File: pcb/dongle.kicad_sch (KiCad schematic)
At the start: 33 parts, among them J1 USB_A, J2 Conn_01x01_Pin, J3 Conn_01x01_Pin, J4 Conn_01x01_Pin, J5 Conn_01x01_Pin, SW1 SW_Push_45deg, U3 nRF52833_QDxx, Y1 Crystal_GND24, Y2 Crystal_Small

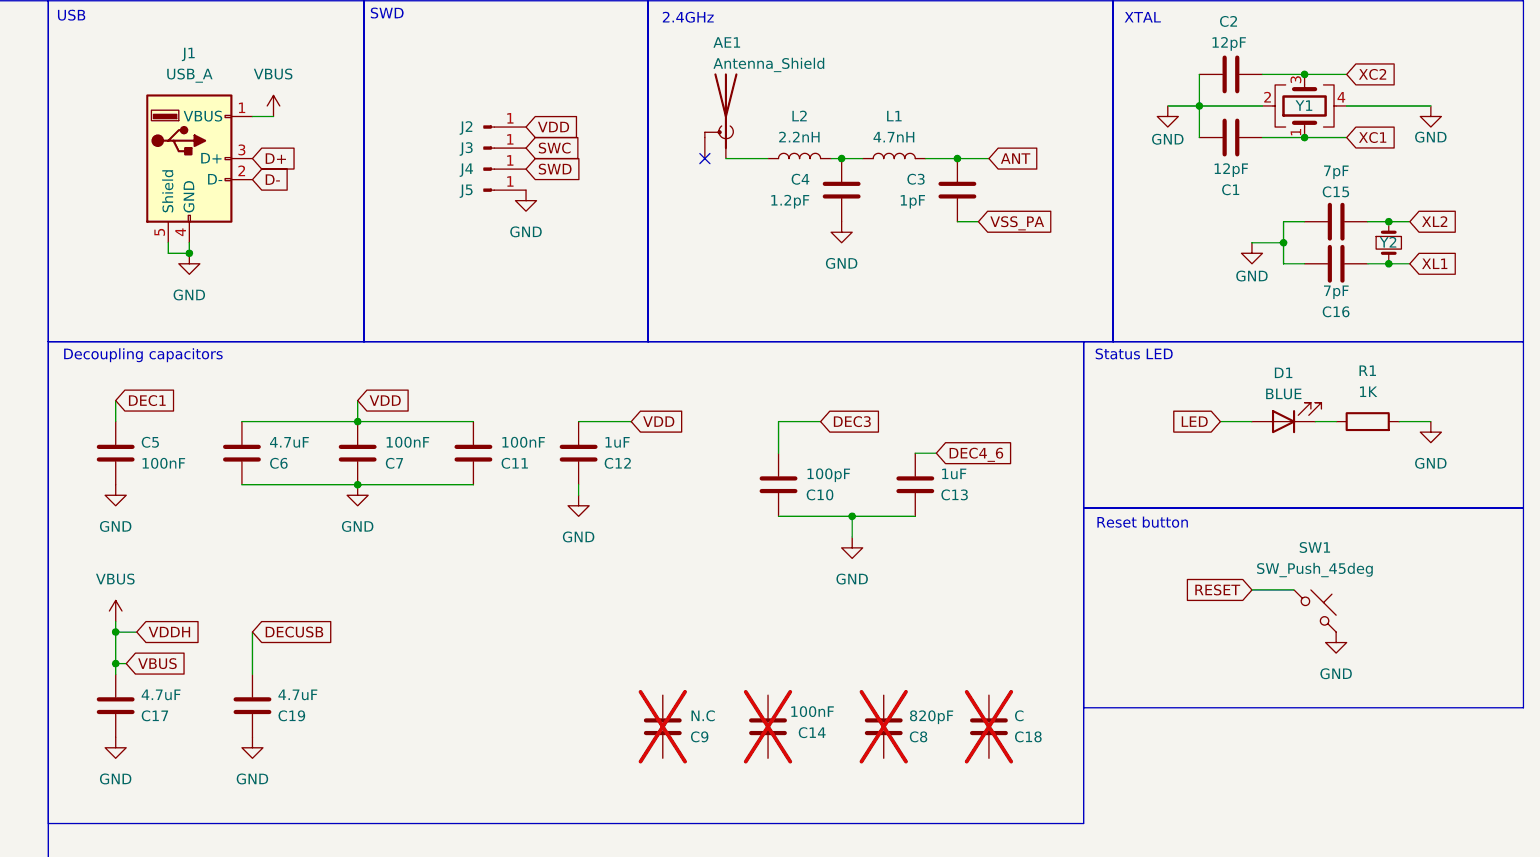
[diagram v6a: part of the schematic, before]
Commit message: update pcb
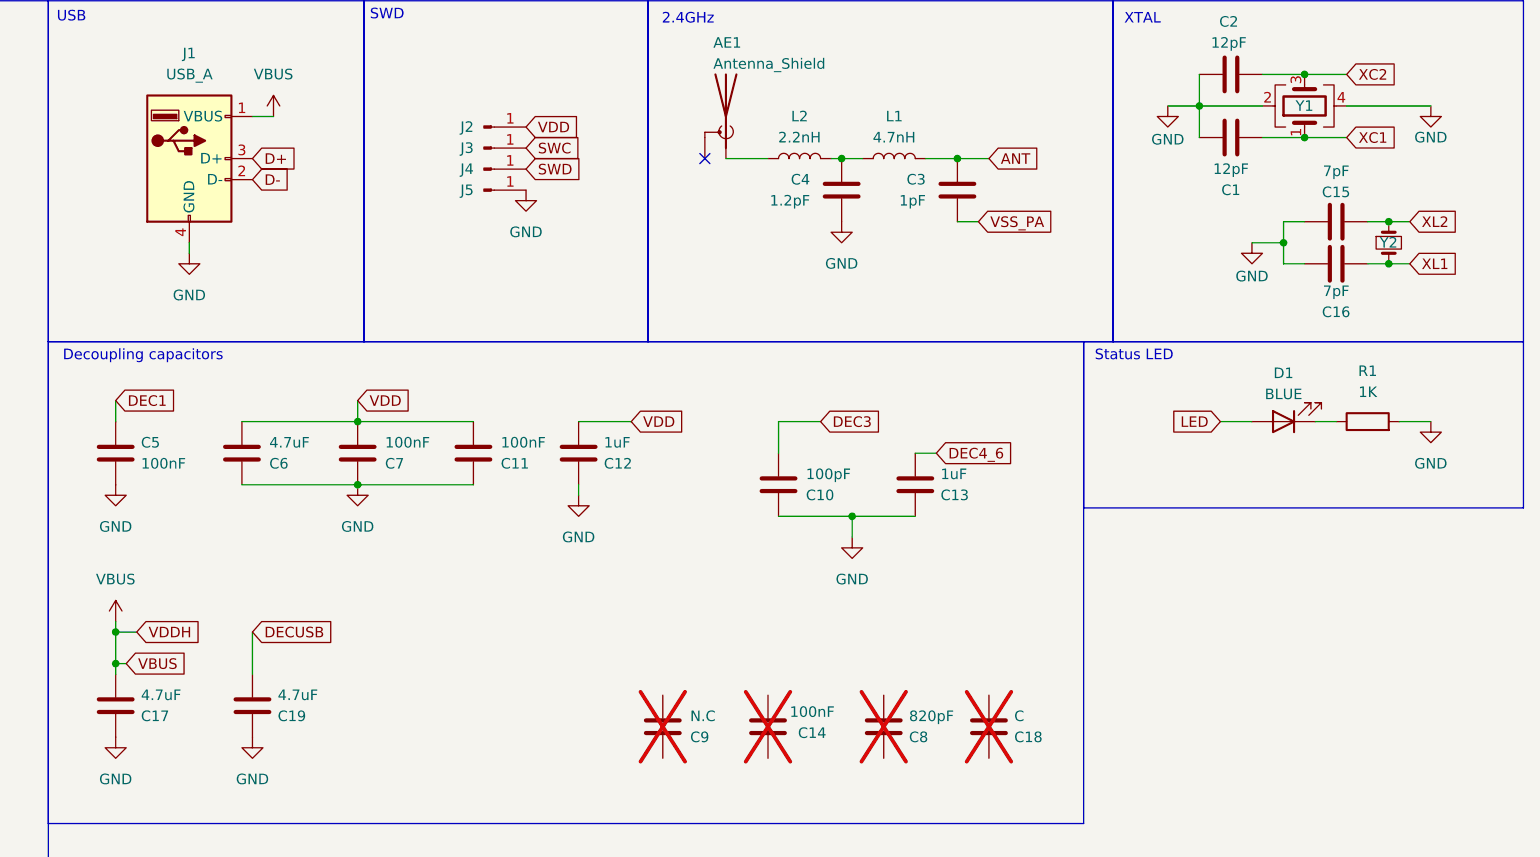
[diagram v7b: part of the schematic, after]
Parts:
- removed SW1: SW_Push_45deg, dongle:SW_SPST_B3U-1000P, symbol dongle:SW_Push_45deg
- J1: footprint dongle:USB_A_Molex_48037-2200_Horizontal -> dongle:USB_A_PCB_Edge_receptacle
- U3: footprint dongle:QFN-40-1EP_5x5mm_P0.4mm_EP3.6x3.6mm_ThermalVias -> dongle:QFN-40-1EP_5x5mm_P0.4mm_EP3.6x3.6mm
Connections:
- net GND: no longer J1.5 (Shield)
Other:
- note removed: "Reset button"
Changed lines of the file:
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@@
 		)
 	)
-	(rectangle
-		(start 231.14 73.914)
-		(end 284.226 98.044)
-		(stroke
-			(width 0)
-			(type default)
-		)
-		(fill
-			(type none)
-		)
-	)
 	(text "USB"
 		(exclude_from_sim no)
@@
 		)
 	)
-	(text "Reset button"
-		(exclude_from_sim no)
-		(at 238.252 75.946 0)
-		(effects
-			(font
-				(size 1.27 1.27)
-			)
-		)
-	)
 	(text "XTAL"
 		(exclude_from_sim no)
@@
 	)
 	(junction
-		(at 123.19 43.18)
-		(diameter 0)
-		(color 0 0 0 0)
-	)
-	(junction
 		(at 267.97 39.37)
 		(diameter 0)
@@
 	(wire
 		(pts
-			(xy 120.65 43.18) (xy 123.19 43.18)
-		)
-		(stroke
-			(width 0)
-			(type default)
-		)
-	)
-	(wire
-		(pts
 			(xy 245.11 25.4) (xy 252.73 25.4)
 		)
@@
 	(wire
 		(pts
-			(xy 251.46 83.82) (xy 256.54 83.82)
-		)
-		(stroke
-			(width 0)
-			(type default)
-		)
-	)
-	(wire
-		(pts
 			(xy 187.96 31.75) (xy 193.04 31.75)
 		)
@@
 	(wire
 		(pts
-			(xy 120.65 41.91) (xy 120.65 43.18)
-		)
-		(stroke
-			(width 0)
-			(type default)
-		)
-	)
-	(wire
-		(pts
 			(xy 115.57 92.71) (xy 114.3 92.71)
 		)
@@
 		)
 	)
-	(global_label "RESET"
-		(shape input)
-		(at 251.46 83.82 180)
-		(fields_autoplaced yes)
-		(effects
-			(font
-				(size 1.27 1.27)
-			)
-			(justify right)
-		)
-		(property "Intersheetrefs" "${INTERSHEET_REFS}"
-			(at 242.7297 83.82 0)
-			(effects
-				(font
-					(size 1.27 1.27)
-				)
-				(justify right)
-				(hide yes)
-			)
-		)
-	)
 	(global_label "VDD"
 		(shape input)
@@
 	)
 	(symbol
-		(lib_id "dongle:SW_Push_45deg")
-		(at 259.08 86.36 0)
-		(unit 1)
-		(exclude_from_sim no)
-		(in_bom yes)
-		(on_board yes)
-		(dnp no)
-		(fields_autoplaced yes)
-		(property "Reference" "SW1"
-			(at 259.08 78.74 0)
-			(effects
-				(font
-					(size 1.27 1.27)
-				)
-			)
-		)
-		(property "Value" "SW_Push_45deg"
-			(at 259.08 81.28 0)
-			(effects
-				(font
-					(size 1.27 1.27)
-				)
-			)
-		)
-		(property "Footprint" "dongle:SW_SPST_B3U-1000P"
-			(at 259.08 86.36 0)
-			(effects
-				(font
-					(size 1.27 1.27)
-				)
-				(hide yes)
-			)
-		)
-		(property "Datasheet" "~"
-			(at 259.08 86.36 0)
-			(effects
-				(font
-					(size 1.27 1.27)
-				)
-				(hide yes)
-			)
-		)
-		(property "Description" "Push button switch, normally open, two pins, 45° tilted"
-			(at 259.08 86.36 0)
-			(effects
-				(font
-					(size 1.27 1.27)
-				)
-				(hide yes)
-			)
-		)
-		(pin "2"
-		)
-		(pin "1"
-		)
-		(instances
-			(project ""
-				(path "/81b8789c-509b-48aa-aabd-6327c54a25df"
-					(reference "SW1")
-					(unit 1)
-				)
-			)
-		)
-	)
-	(symbol
 		(lib_id "PNCATEHO_lowair:C")
 		(at 170.18 67.31 0)
@@
 	)
 	(symbol
-		(lib_id "Library:GND")
-		(at 261.62 88.9 0)
-		(unit 1)
-		(exclude_from_sim no)
-		(in_bom yes)
-		(on_board yes)
-		(dnp no)
-		(fields_autoplaced yes)
-		(property "Reference" "#PWR05"
-			(at 261.62 95.25 0)
-			(effects
-				(font
-					(size 1.27 1.27)
-				)
-				(hide yes)
-			)
-		)
-		(property "Value" "GND"
-			(at 261.62 93.98 0)
-			(effects
-				(font
-					(size 1.27 1.27)
-				)
-			)
-		)
-		(property "Footprint" ""
-			(at 261.62 88.9 0)
-			(effects
-				(font
-					(size 1.27 1.27)
-				)
-				(hide yes)
-			)
-		)
-		(property "Datasheet" ""
-			(at 261.62 88.9 0)
-			(effects
-				(font
-					(size 1.27 1.27)
-				)
-				(hide yes)
-			)
-		)
-		(property "Description" "Global ground symbol"
-			(at 261.62 98.298 0)
-			(effects
-				(font
-					(size 1.27 1.27)
-				)
-				(hide yes)
-			)
-		)
-		(pin "1"
-		)
-		(instances
-			(project "dongle"
-				(path "/81b8789c-509b-48aa-aabd-6327c54a25df"
-					(reference "#PWR05")
-					(unit 1)
-				)
-			)
-		)
-	)
-	(symbol
 		(lib_id "PNCATEHO_lowair:VBUS")
 		(at 114.3 87.63 0)
@@
 			)
 		)
-		(property "Footprint" "dongle:USB_A_Molex_48037-2200_Horizontal"
+		(property "Footprint" "dongle:USB_A_PCB_Edge_receptacle"
 			(at 127 33.02 0)
 			(effects
@@
 		(pin "1"
 		)
-		(pin "5"
-		)
 		(instances
 			(project ""
@@
 			)
 		)
-		(property "Footprint" "dongle:QFN-40-1EP_5x5mm_P0.4mm_EP3.6x3.6mm_ThermalVias"
+		(property "Footprint" "dongle:QFN-40-1EP_5x5mm_P0.4mm_EP3.6x3.6mm"
 			(at 59.69 180.34 0)
 			(effects

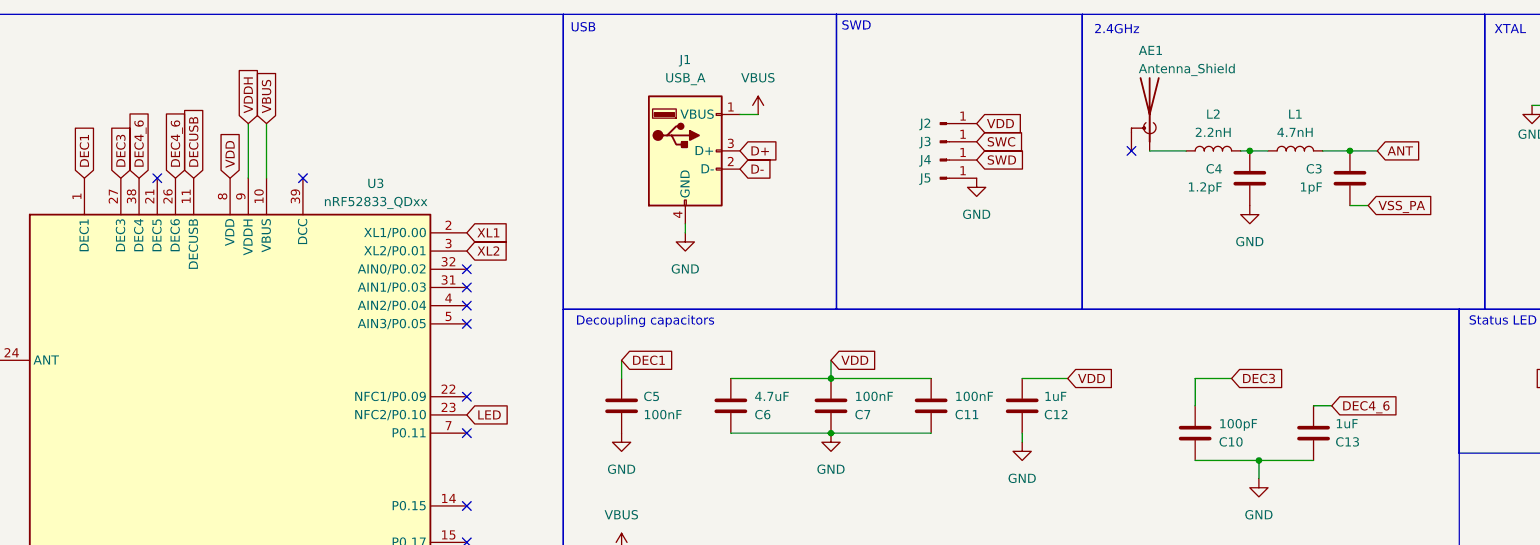
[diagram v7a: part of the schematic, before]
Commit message: update footprint
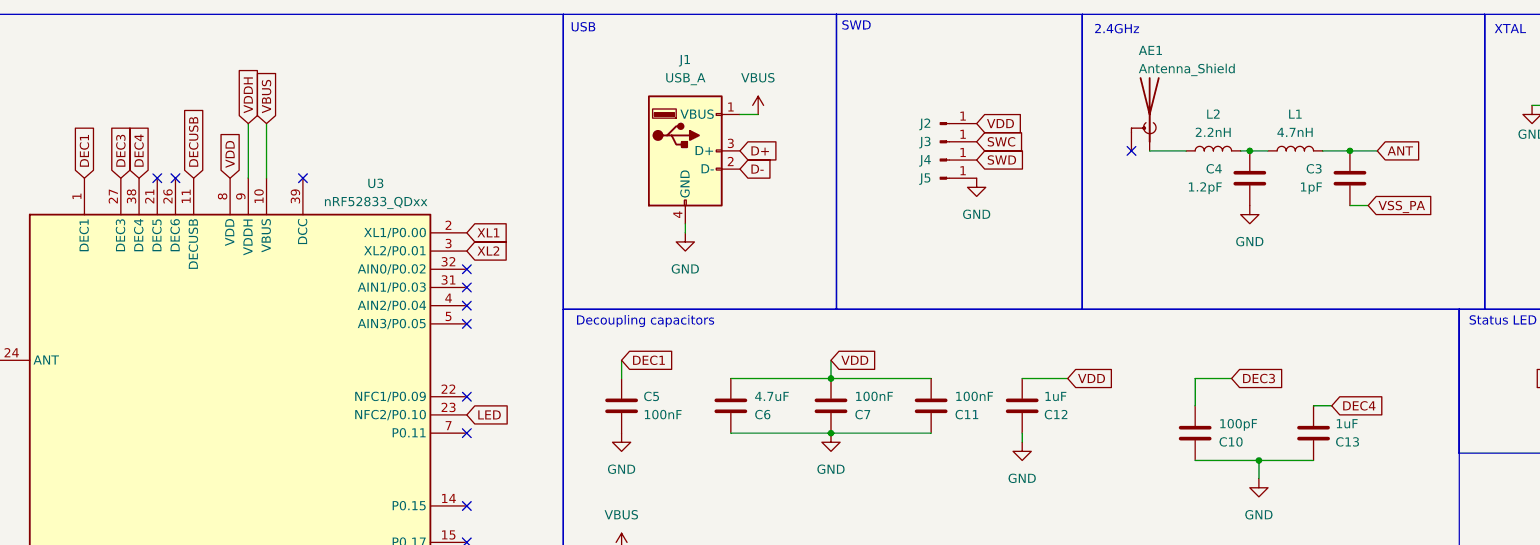
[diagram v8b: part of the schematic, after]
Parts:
- J1: footprint dongle:USB_A_PCB_Edge_receptacle -> dongle:USB_A_PCB_Edge
- J2, J3, J4: footprint dongle:TestPoint_Pad_D1.0mm -> dongle:TestPoint_Pad_R
- J5: footprint dongle:TestPoint_Pad_1.0x1.0mm -> dongle:TestPoint_Pad
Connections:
- net DEC4_6 renamed DEC4
- net DEC4: no longer U3.26 (DEC6)
- no-connect marks 17 -> 18
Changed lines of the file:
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@@
 	)
 	(no_connect
+		(at 52.07 35.56)
+	)
+	(no_connect
 		(at 185.42 31.75)
 	)
@@
 		)
 	)
-	(global_label "DEC4_6"
+	(global_label "DEC4"
 		(shape input)
 		(at 46.99 35.56 90)
@@
 		)
 		(property "Intersheetrefs" "${INTERSHEET_REFS}"
-			(at 46.99 25.4992 90)
+			(at 46.99 27.6763 90)
 			(effects
 				(font
@@
 		)
 	)
-	(global_label "DEC4_6"
+	(global_label "DEC4"
 		(shape input)
 		(at 213.36 67.31 0)
@@
 		)
 		(property "Intersheetrefs" "${INTERSHEET_REFS}"
-			(at 223.4208 67.31 0)
+			(at 221.2437 67.31 0)
 			(effects
 				(font
@@
 		)
 	)
-	(global_label "DEC4_6"
-		(shape input)
-		(at 52.07 35.56 90)
-		(fields_autoplaced yes)
-		(effects
-			(font
-				(size 1.27 1.27)
-			)
-			(justify left)
-		)
-		(property "Intersheetrefs" "${INTERSHEET_REFS}"
-			(at 52.07 25.4992 90)
-			(effects
-				(font
-					(size 1.27 1.27)
-				)
-				(justify left)
-				(hide yes)
-			)
-		)
-	)
 	(global_label "VDDH"
 		(shape input)
@@
 			)
 		)
-		(property "Footprint" "dongle:TestPoint_Pad_1.0x1.0mm"
+		(property "Footprint" "dongle:TestPoint_Pad"
 			(at 158.75 35.56 0)
 			(effects
@@
 			)
 		)
-		(property "Footprint" "dongle:TestPoint_Pad_D1.0mm"
+		(property "Footprint" "dongle:TestPoint_Pad_R"
 			(at 158.75 33.02 0)
 			(effects
@@
 			)
 		)
-		(property "Footprint" "dongle:TestPoint_Pad_D1.0mm"
+		(property "Footprint" "dongle:TestPoint_Pad_R"
 			(at 158.75 30.48 0)
 			(effects
@@
 			)
 		)
-		(property "Footprint" "dongle:USB_A_PCB_Edge_receptacle"
+		(property "Footprint" "dongle:USB_A_PCB_Edge"
 			(at 127 33.02 0)
 			(effects
@@
 			)
 		)
-		(property "Footprint" "dongle:TestPoint_Pad_D1.0mm"
+		(property "Footprint" "dongle:TestPoint_Pad_R"
 			(at 158.75 27.94 0)
 			(effects
